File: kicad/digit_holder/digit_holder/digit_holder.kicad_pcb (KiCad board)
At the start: 2 copper layers, 25.4 x 31.8 mm, 3 parts, among them J1 Conn_01x07_Male, J2 Conn_01x08_Male

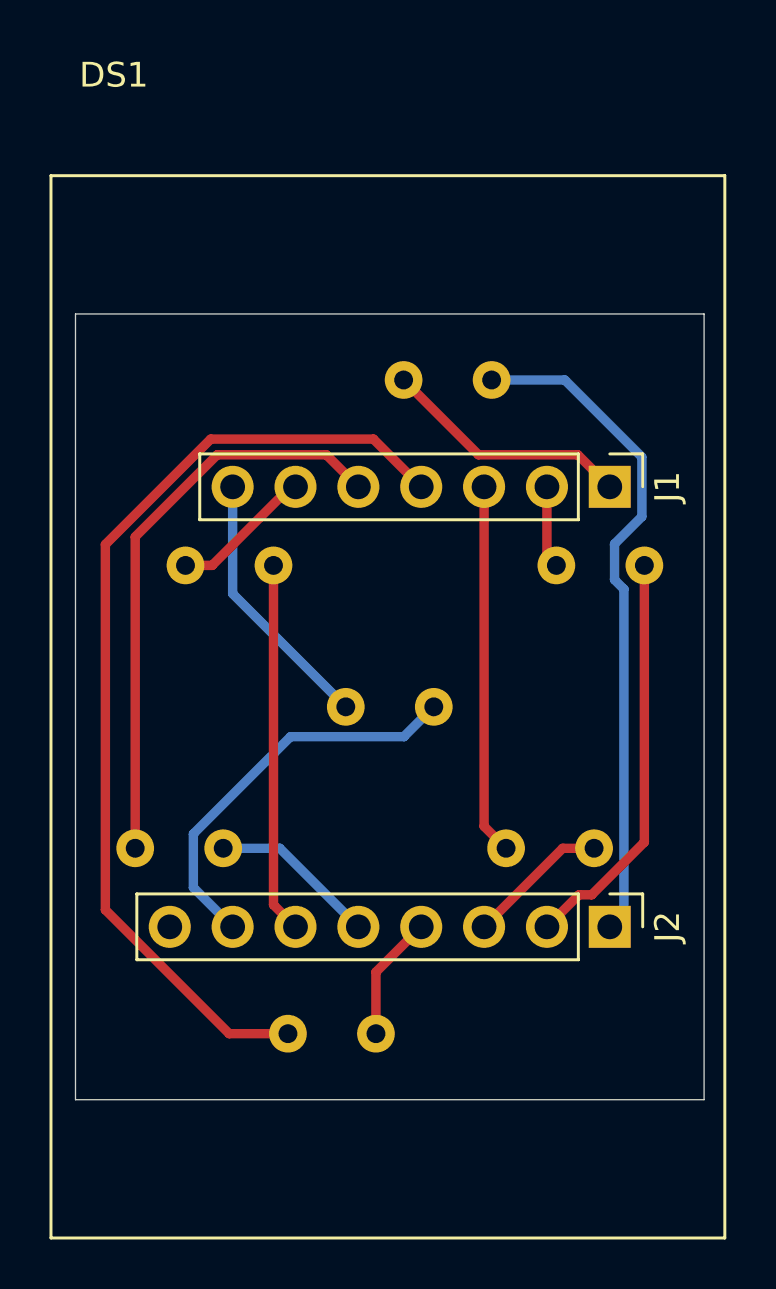
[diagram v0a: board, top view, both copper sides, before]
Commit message: update pcb
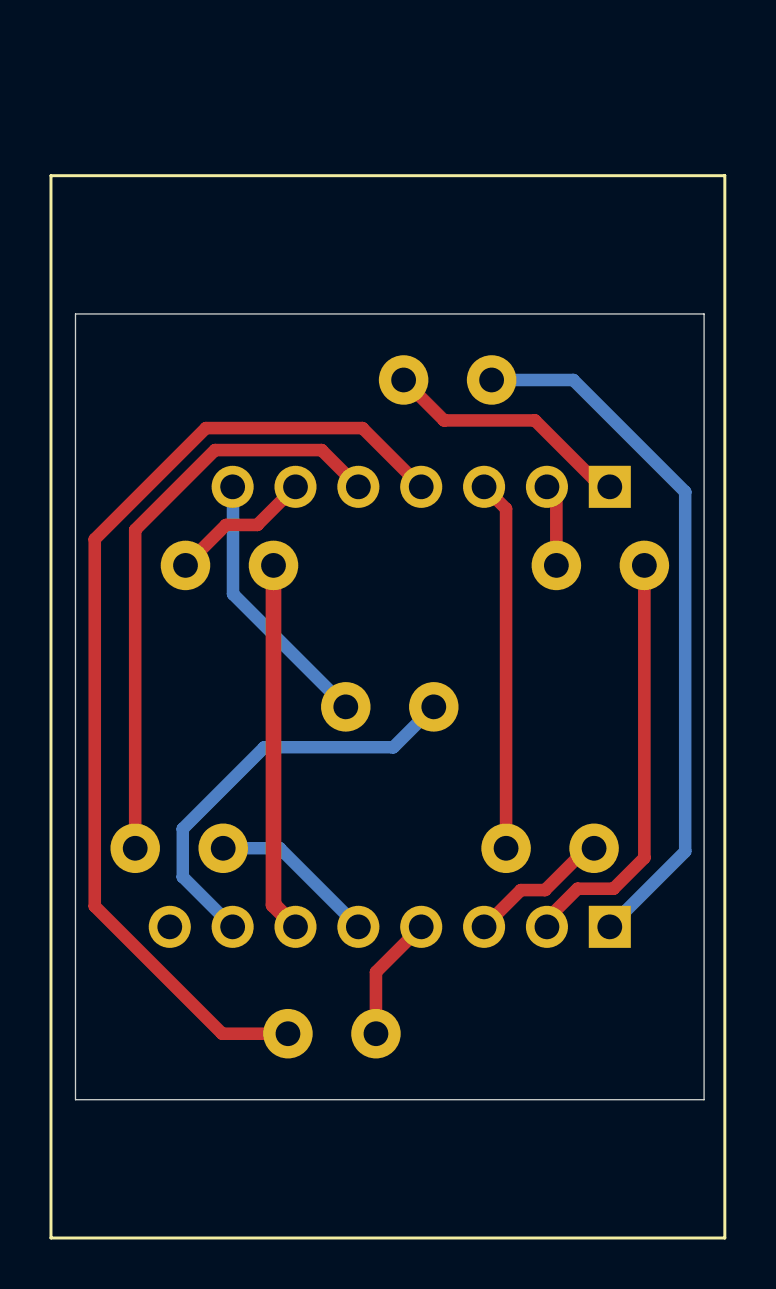
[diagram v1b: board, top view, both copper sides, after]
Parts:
- J1, J2: moved to B.Cu
- turned J1 to 90 degrees
- turned J2 to 90 degrees
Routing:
- net Net-(DS1-PadD1): track 39.5 -> 40.8 mm
- net Net-(DS1-PadA2): track 28.0 -> 29.3 mm
- net Net-(DS1-PadB2): track 16.5 -> 17.5 mm
- net Net-(DS1-PadG2): track 16.3 -> 17.0 mm
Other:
- net class Default: clearance 0.254 -> 0.381
- rule trace_clearance: 0.254 -> 0.381
- board text added: "Reset"
- board text added: "Set"
